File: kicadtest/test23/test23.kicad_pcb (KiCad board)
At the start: 2 copper layers, 6 parts

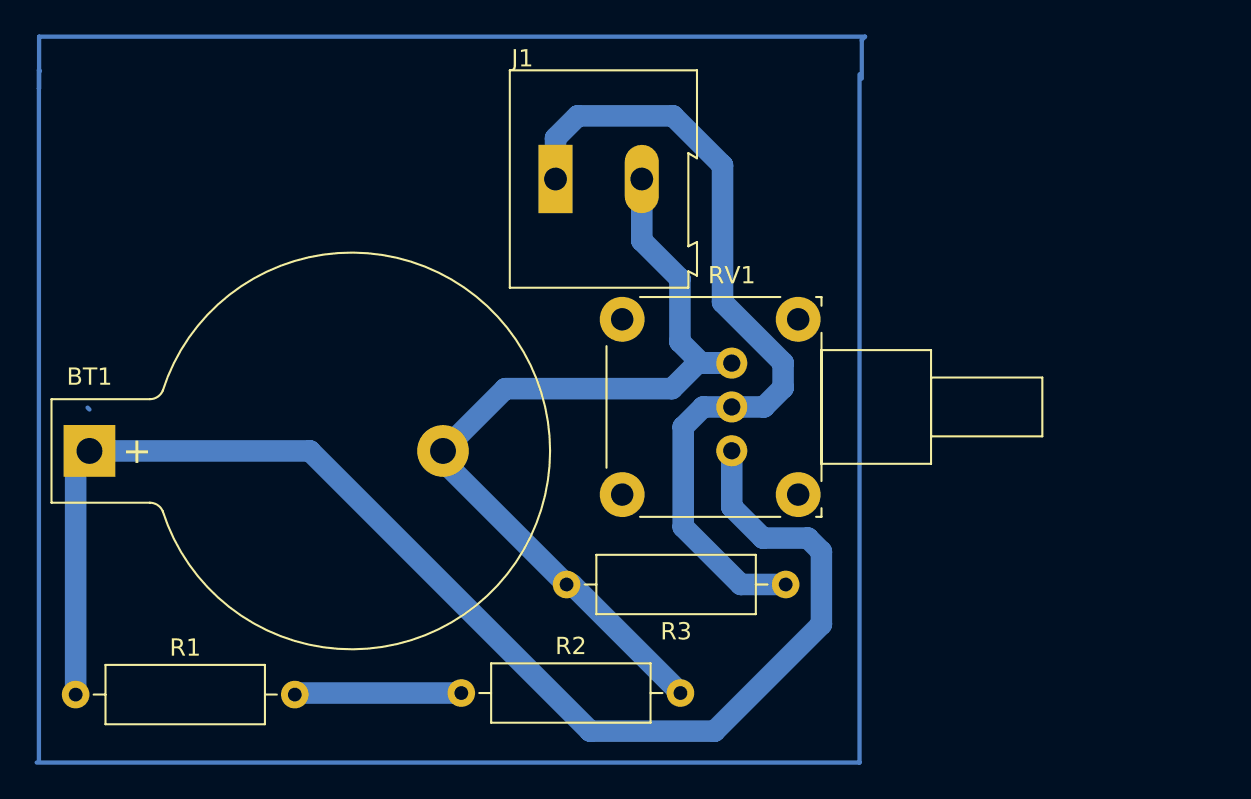
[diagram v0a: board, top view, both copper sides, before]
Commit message: petite modif
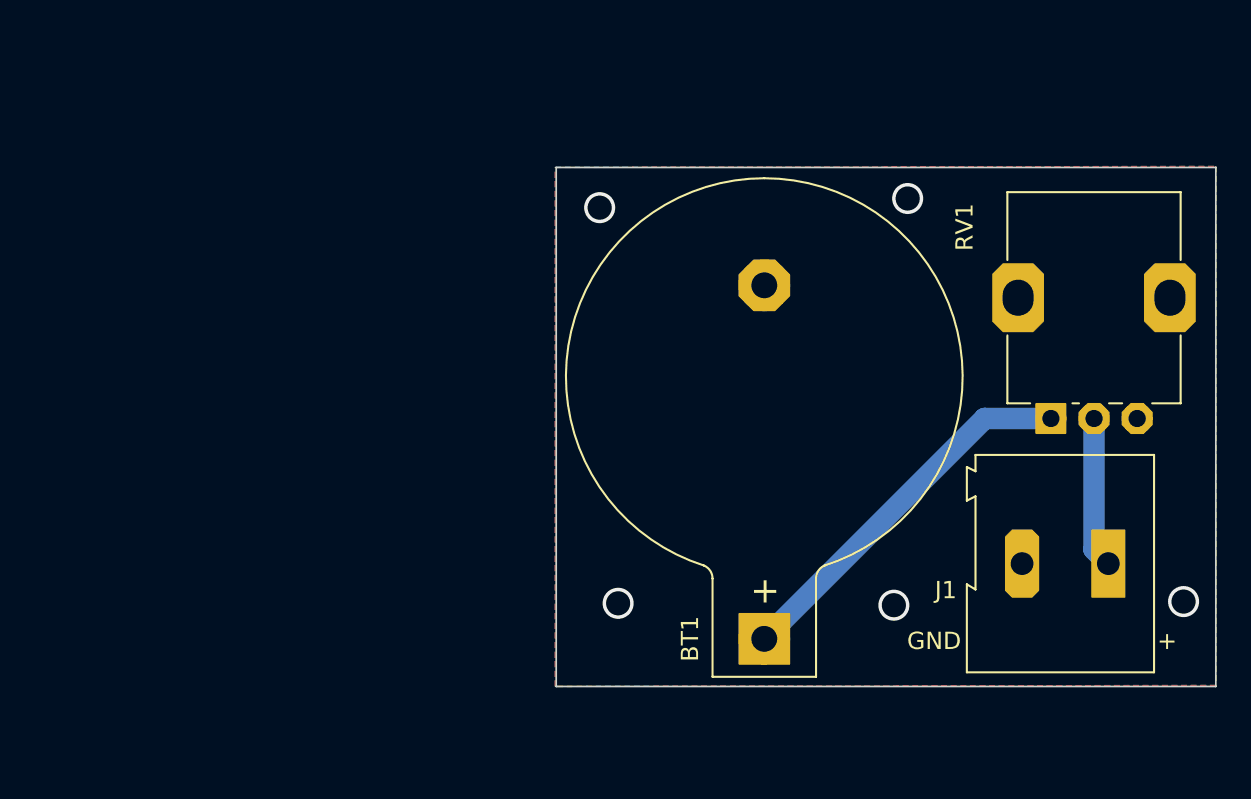
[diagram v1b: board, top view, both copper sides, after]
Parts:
- removed R1, R2, R3: 100k, Resistor_THT:R_Axial_DIN0309_L9.0mm_D3.2mm_P12.70mm_Horizontal
- BT1: value 5V -> 5
- RV1: footprint Potentiometer_THT:Potentiometer_Vishay_148E-149E_Single_Horizontal -> Potentiometer_THT:Potentiometer_Alps_RK09K_Single_Vertical
- moved BT1 40.6 mm to (147.5, 78.0), turned to 90 degrees
- moved J1 39.0 mm to (167.4, 73.6), turned to 180 degrees
- moved RV1 18.6 mm to (164.1, 65.2), turned to 90 degrees
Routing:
- net (no net): track 181.1 -> 0.00 mm
- net V1: track 80.1 -> 21.9 mm
- net VGND: track 53.0 -> 0.00 mm, vias 0 -> 5
- net V2: track 48.0 -> 8.75 mm
- net V3: track 9.81 -> 0.00 mm
- added copper zone on B.Cu, net VGND
- added copper zone on F.Cu, net VGND
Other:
- board outline added: 38.2 x 30.1 mm
- board text added: "+"
- board text added: "GND"
